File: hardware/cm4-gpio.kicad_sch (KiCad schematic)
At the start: 6 parts, among them J2 DF40C-100DP-0.4V_51_

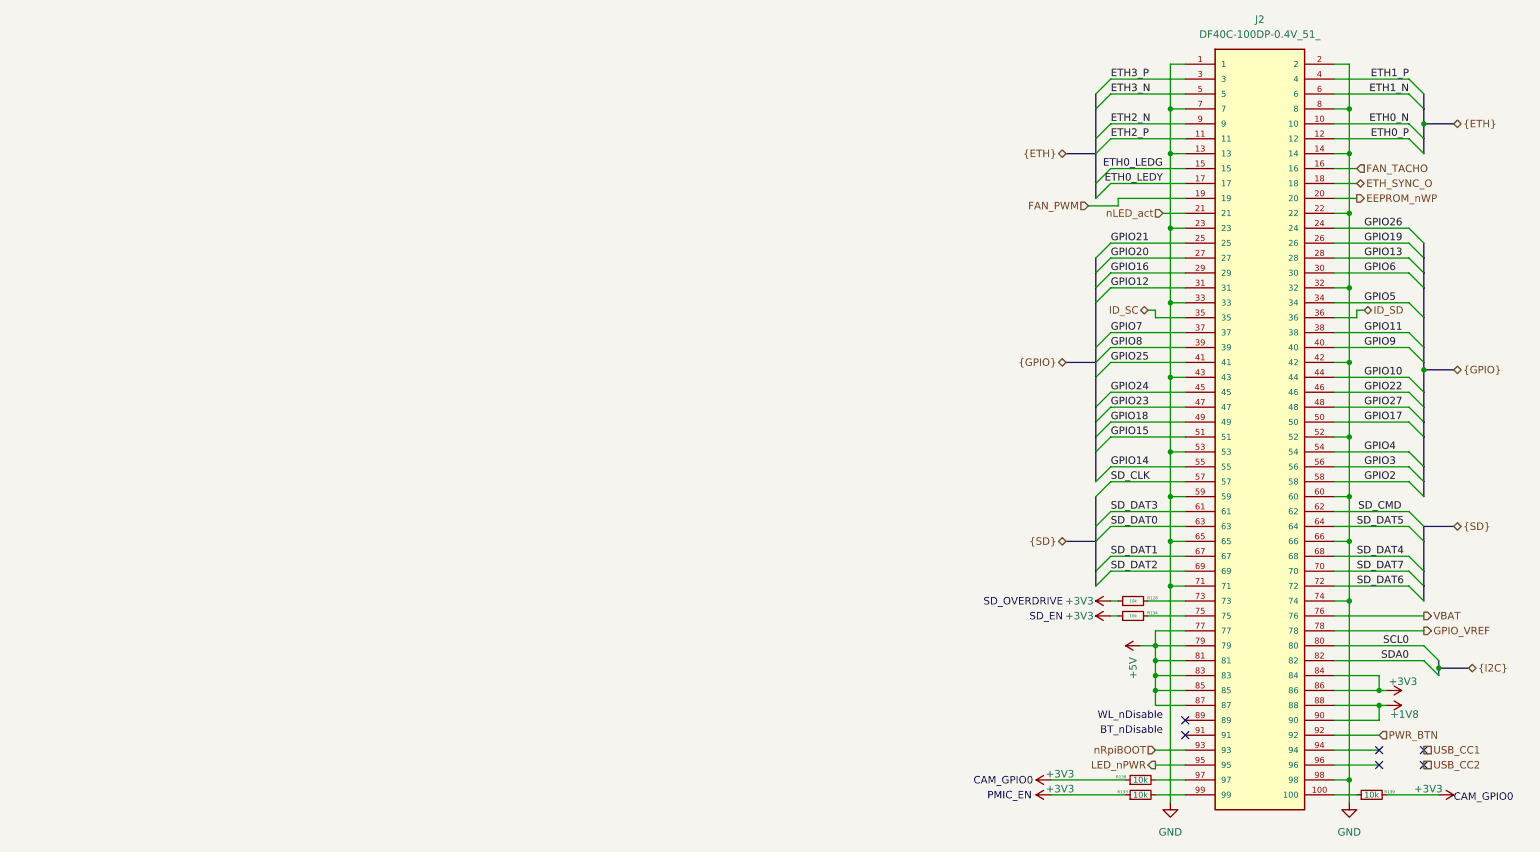
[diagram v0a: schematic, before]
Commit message: Cleanup
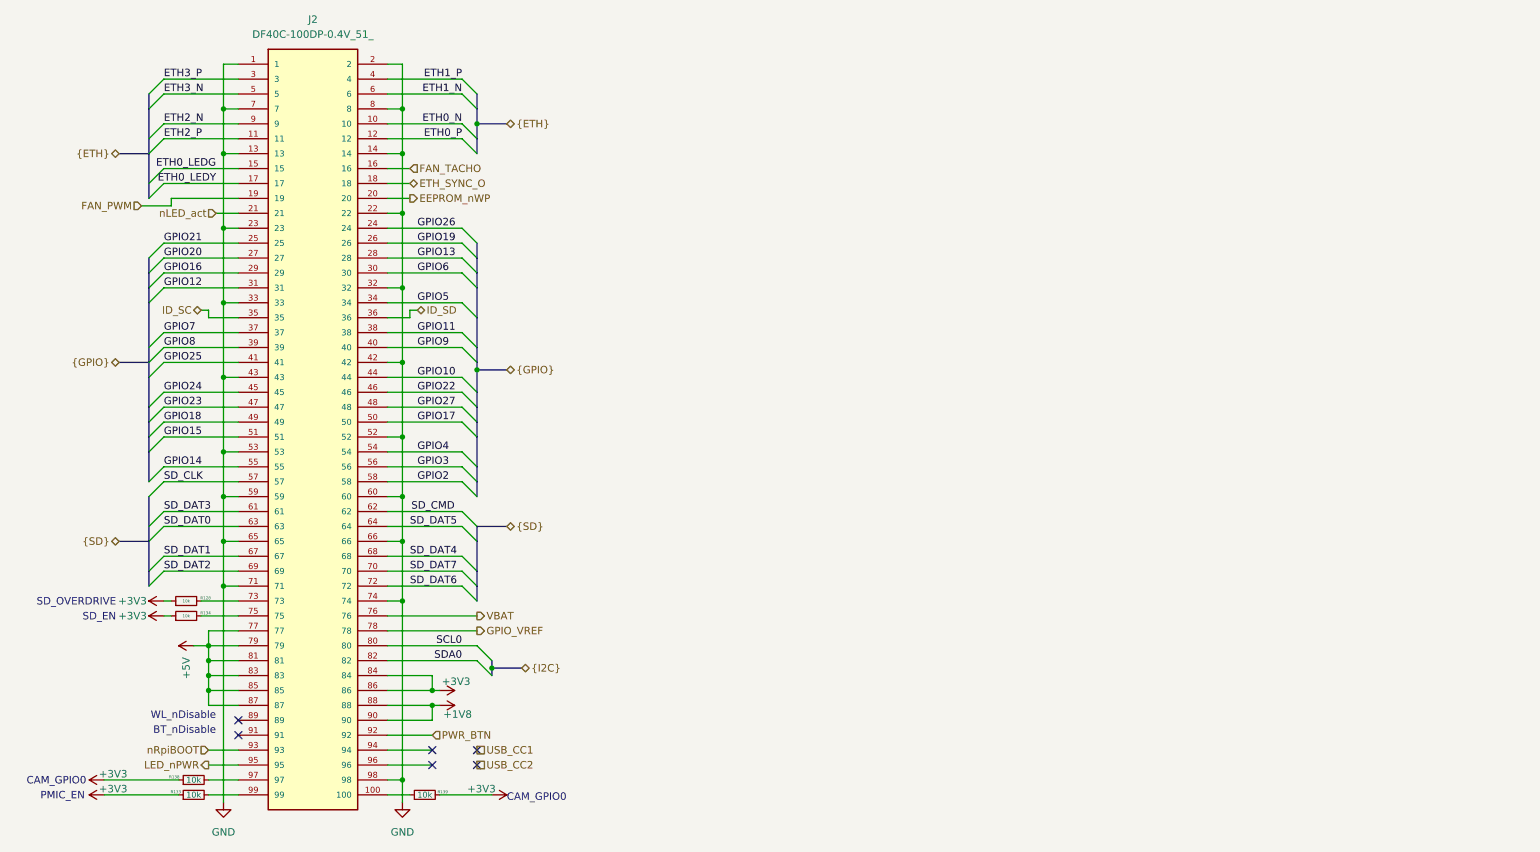
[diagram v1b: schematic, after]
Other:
- moved on the sheet: J2, R128, R133, R134, R138, R139
